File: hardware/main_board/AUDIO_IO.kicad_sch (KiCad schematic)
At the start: 0 parts

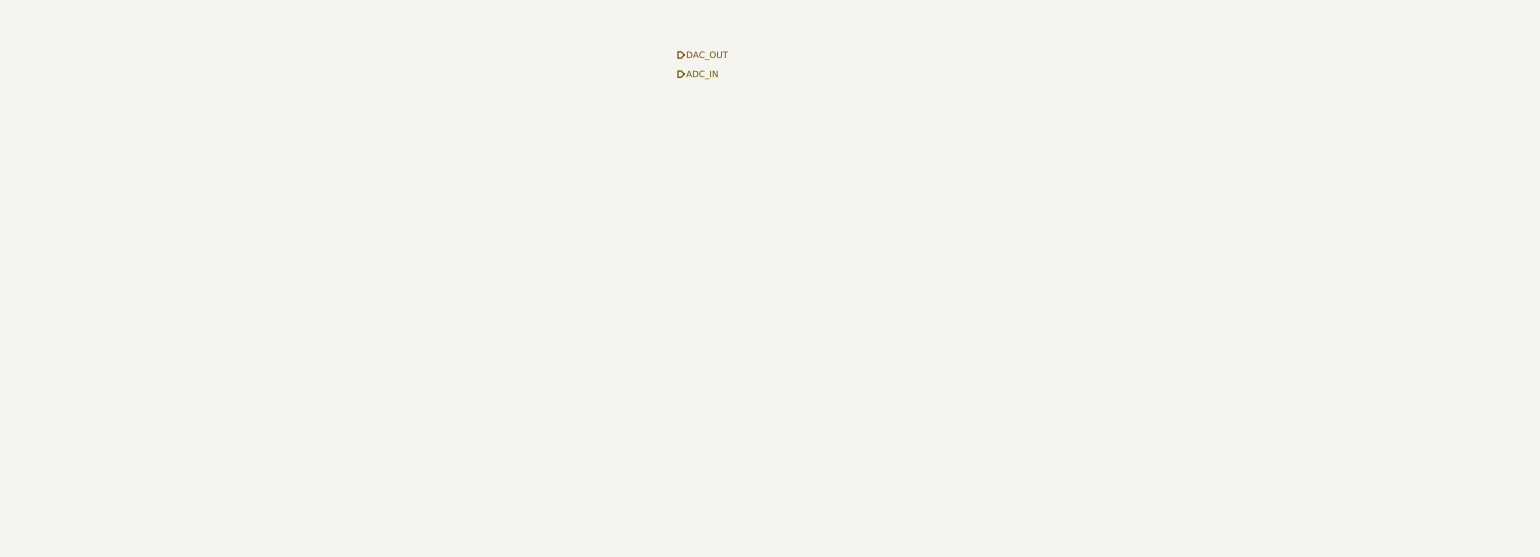
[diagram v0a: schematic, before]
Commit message: drew schematic
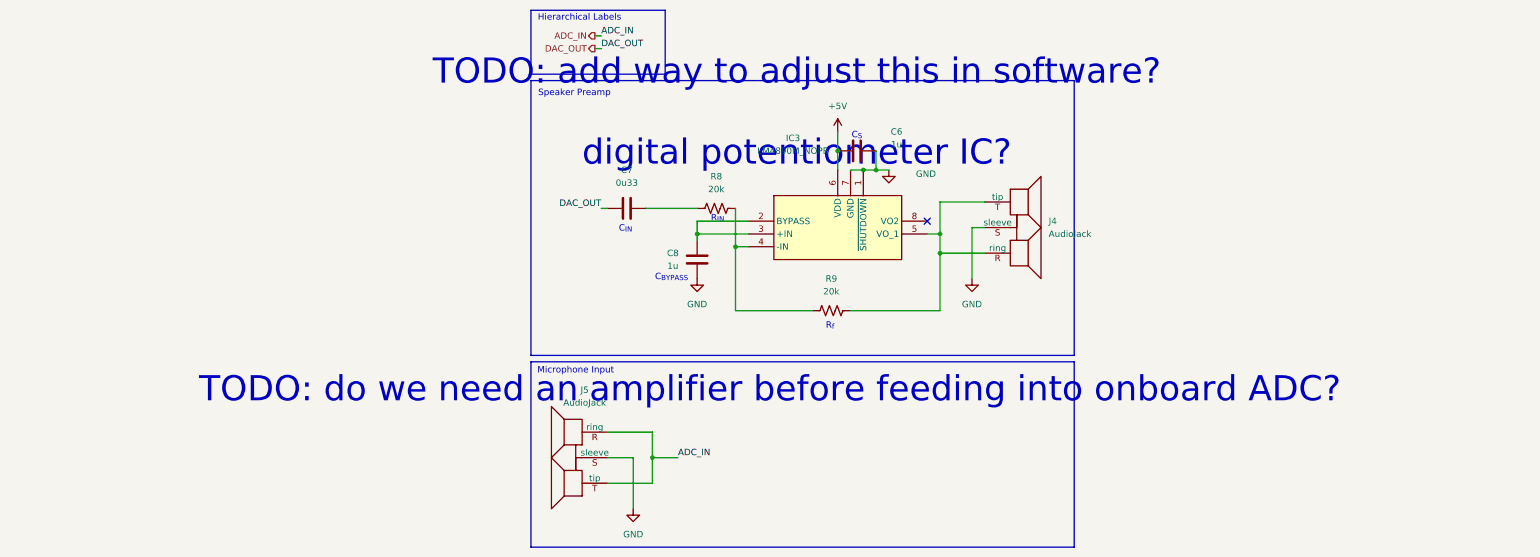
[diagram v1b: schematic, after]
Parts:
- added C6, C8: 1u, Capacitor_SMD:C_0805_2012Metric, symbol ECE445L:C
- added C7: 0u33, Capacitor_SMD:C_0805_2012Metric, symbol ECE445L:C
- added IC3: LM4890M_NOPB, 445L:ti_LM4890M_NOPB, symbol ECE445L:LM4890M_NOPB
- added J4, J5: AudioJack, 445L:Jack_3.5mm_CUI_SJ1-3523N_Horizontal, symbol ECE445L:HeadphoneJack
- added R8, R9: 20k, Resistor_SMD:R_0805_2012Metric, symbol Device:R_US
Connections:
- net ADC_IN: now also J5.R (ring), J5.T (tip)
- net DAC_OUT: now also C7.1
- new net: C7.2, R8.1
- new net: C8.1, IC3.2 (BYPASS), IC3.3 (+IN)
- new net: IC3.4 (-IN), R8.2, R9.1
- new net: IC3.5 (VO_1), J4.R (ring), J4.T (tip), R9.2
- new net +5V: C6.2, IC3.6 (VDD)
- new net GND: C6.1, C8.2, IC3.1 (~{SHUTDOWN}), IC3.7 (GND), J4.S (sleeve), J5.S (sleeve)
- no-connect marks 0 -> 1
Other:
- note added: "C_{BYPASS}"
- note added: "C_{IN}"
- note added: "C_{S}"
- note added: "Hierarchical Labels"
- note added: "Microphone Input"
- note added: "R_{IN}"
- note added: "R_{f}"
- note added: "Speaker Preamp"
- note added: "TODO: add way to adjust this in software? digital potentiometer IC?"
- note added: "TODO: do we need an amplifier before feeding into onboard ADC?"
